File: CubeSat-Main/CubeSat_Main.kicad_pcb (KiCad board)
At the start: 2 copper layers, 92 x 92 mm, 25 parts, among them J1 Conn_01x03_Pin, J2 Conn_01x08_Socket, U1 STM32F411CEU6 - BlackPill, U2 LORA E220-900T22D, U3 BNO055, U4 LM35-LP, U5 GPS_NEO6M

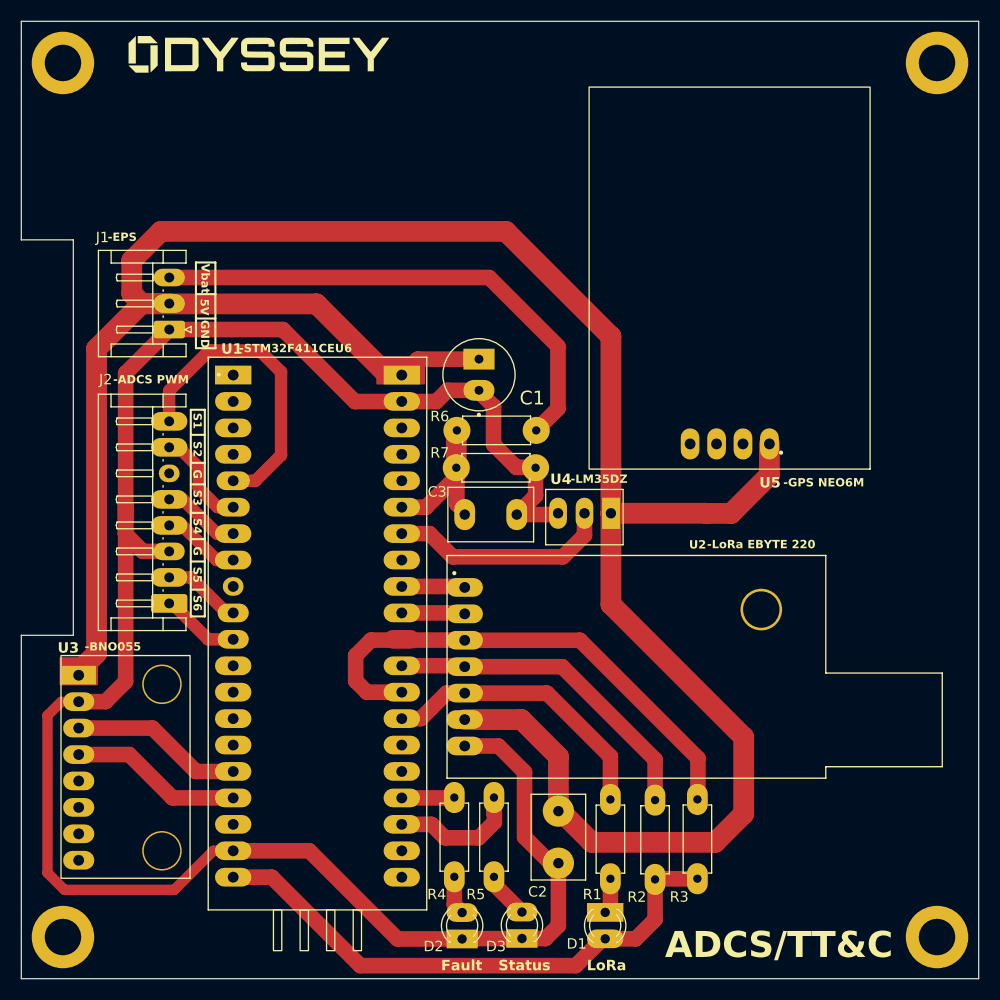
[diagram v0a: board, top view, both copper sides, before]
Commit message: small changes only
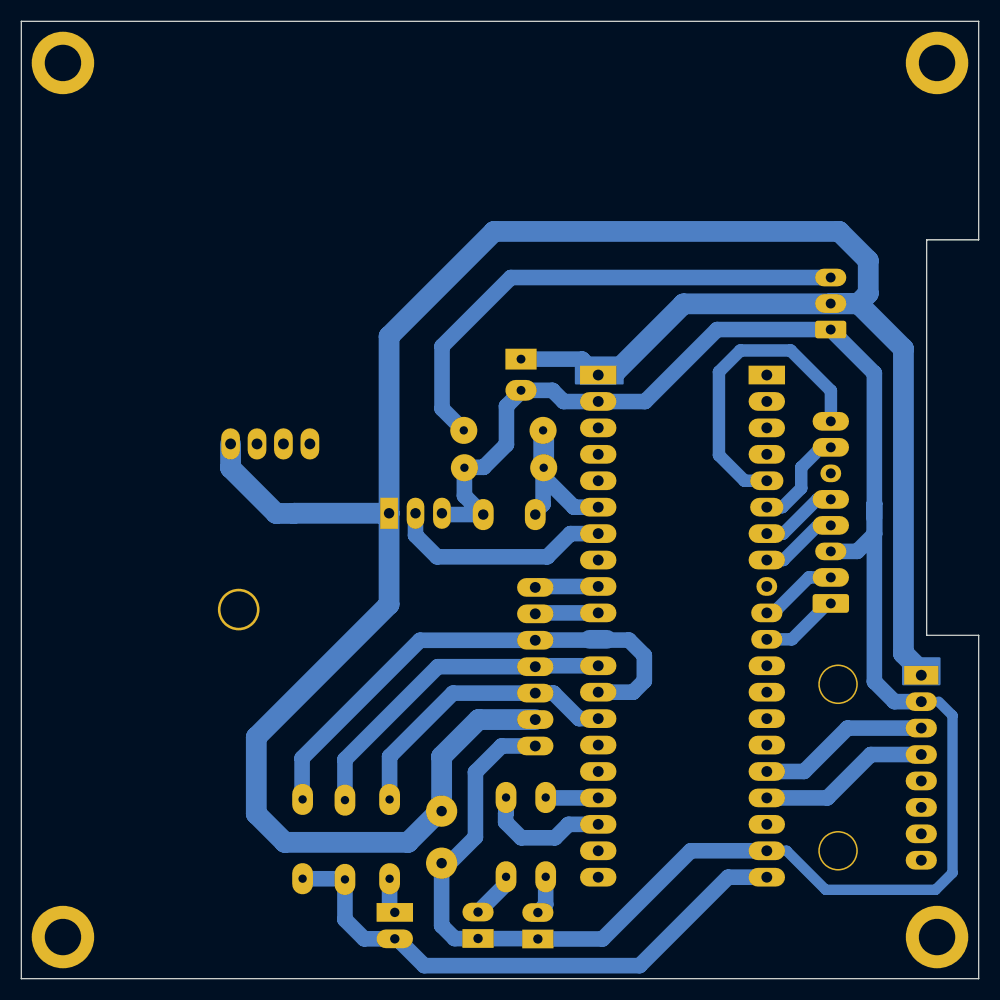
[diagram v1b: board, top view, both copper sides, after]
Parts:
- C1, C2, C3, D1, D2, D3, G***, J1, J2, R1, R2, R3, R4, R5, R6, R7, REF** (x4), U1, U2, U3, U4, U5: moved to B.Cu
- moved REF** 84.0 mm to (4.00, -4.00), turned to 180 degrees
- moved REF** 84.0 mm to (88.0, -4.00), turned to 180 degrees
- moved REF** 84.0 mm to (4.00, -88.0), turned to 180 degrees
- moved REF** 84.0 mm to (88.0, -88.0), turned to 180 degrees
- moved U3 72.0 mm to (82.0, -20.3), turned to 0 degrees
- moved J2 63.6 mm to (77.8, -36.1)
- moved J1 63.6 mm to (77.8, -62.4)
- moved G*** 46.2 mm to (69.1, -88.8), turned to 180 degrees
- moved U5 43.9 mm to (24.1, -66.9), turned to 0 degrees
- moved R3 37.9 mm to (27.0, -17.2)
- moved U1 35.1 mm to (63.5, -33.5), turned to 180 degrees
- moved R2 29.8 mm to (31.1, -17.2)
- moved U2 26.2 mm to (32.9, -30.0)
- moved R1 21.2 mm to (35.4, -17.2)
- moved D1 20.2 mm to (35.9, -6.37)
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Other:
- outline, holes or cut-outs redrawn
